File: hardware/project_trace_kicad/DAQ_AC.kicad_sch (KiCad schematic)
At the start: 52 parts, among them U301 THS4131IDR, U303 ADS1602, U304 MCP6499T, U305 LM4040DBZ-2.5, U306 LM4040DBZ-4.1

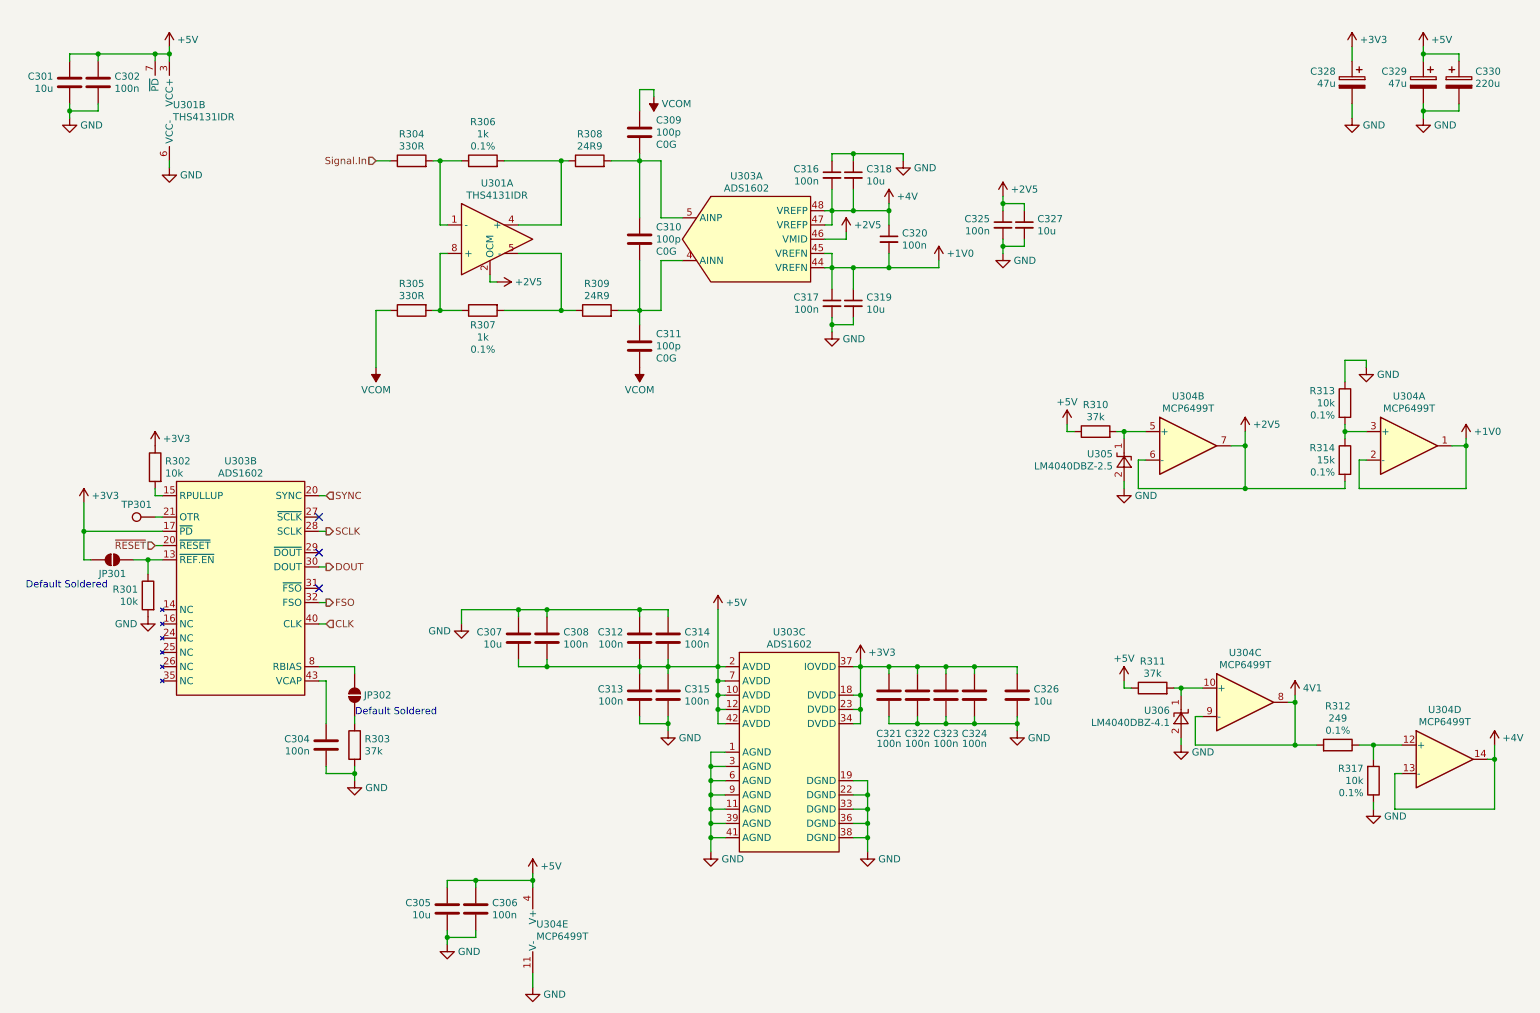
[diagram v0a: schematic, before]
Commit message: Address Review Comments
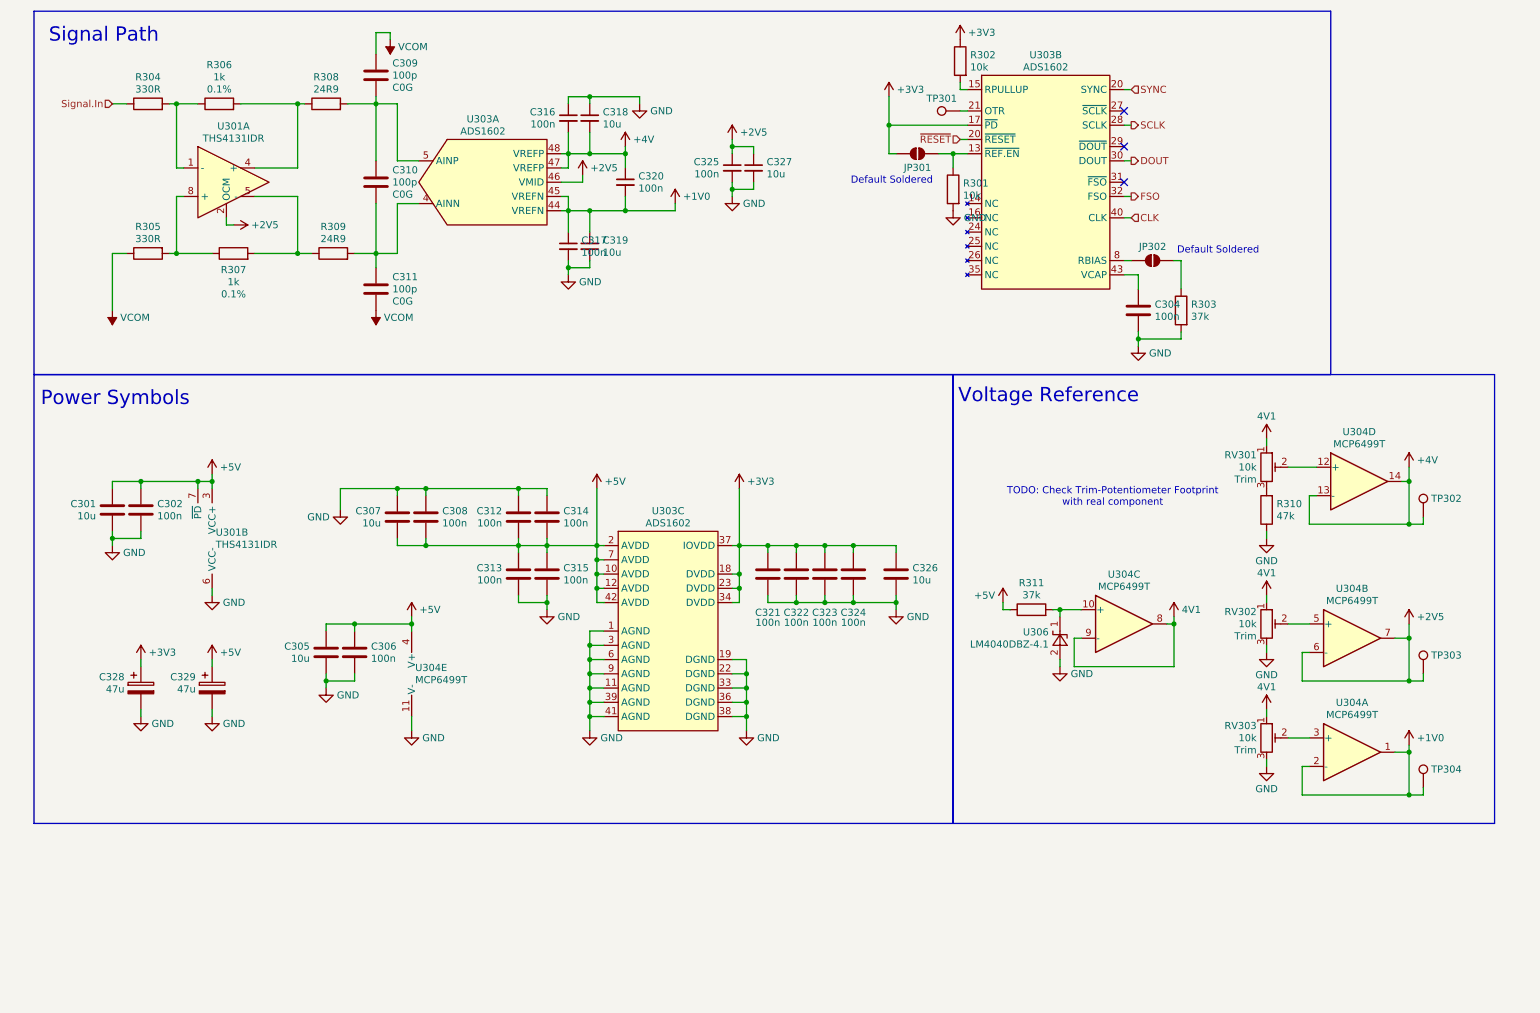
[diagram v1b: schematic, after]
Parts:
- removed C330: 220u, symbol Device:C_Polarized
- removed R312: 249, Resistor_SMD:R_0603_1608Metric_Pad0.98x0.95mm_HandSolder, symbol Device:R
- removed R313, R317: 10k, Resistor_SMD:R_0603_1608Metric_Pad0.98x0.95mm_HandSolder, symbol Device:R
- removed R314: 15k, Resistor_SMD:R_0603_1608Metric_Pad0.98x0.95mm_HandSolder, symbol Device:R
- removed U305: LM4040DBZ-2.5, Package_TO_SOT_SMD:SOT-23_Handsoldering, symbol Reference_Voltage:LM4040DBZ-2.5
- added RV301, RV302, RV303: 10k, Potentiometer_THT:Potentiometer_Bourns_3266W_Vertical, symbol Device:R_Potentiometer_Trim
- added TP302, TP303, TP304: TestPoint, TestPoint:TestPoint_Pad_1.5x1.5mm, symbol Connector:TestPoint
- C328, C329: footprint (none) -> Capacitor_THT:CP_Radial_D6.3mm_P2.50mm
- R310: value 37k -> 47k; footprint Resistor_SMD:R_0603_1608Metric_Pad0.98x0.95mm_HandSolder -> Resistor_THT:R_Axial_DIN0207_L6.3mm_D2.5mm_P10.16mm_Horizontal; DigikeyPN 2019-RN73R1JTTD3702F100CT-ND -> N/A
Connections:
- net +1V0: now also TP304.1
- net +2V5: now also TP303.1
- net +4V: now also TP302.1
- net +5V: no longer R310.1
- net 4V1: now also RV301.1, RV302.1, RV303.1
- net GND: now also R310.1, RV302.3, RV303.3
- net at R310.2: now also RV301.3; no longer U304.5 (+)
- net at U304.3 (+): now also RV303.2
- net at U304.12 (+): now also RV301.2
- new net: RV302.2, U304.5 (+)
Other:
- note added: "Power Symbols"
- note added: "Signal Path"
- note added: "TODO: Check Trim-Potentiometer Footprint with real component"
- note added: "Voltage Reference"
- moved on the sheet: C301, C302, C304, C305, C306, C307, C308, C309, C310, C311, C312, C313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
